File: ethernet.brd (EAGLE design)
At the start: 32.5 x 17 mm, 2 parts, among them CN1 8P8C, CN7 Mini Displayport

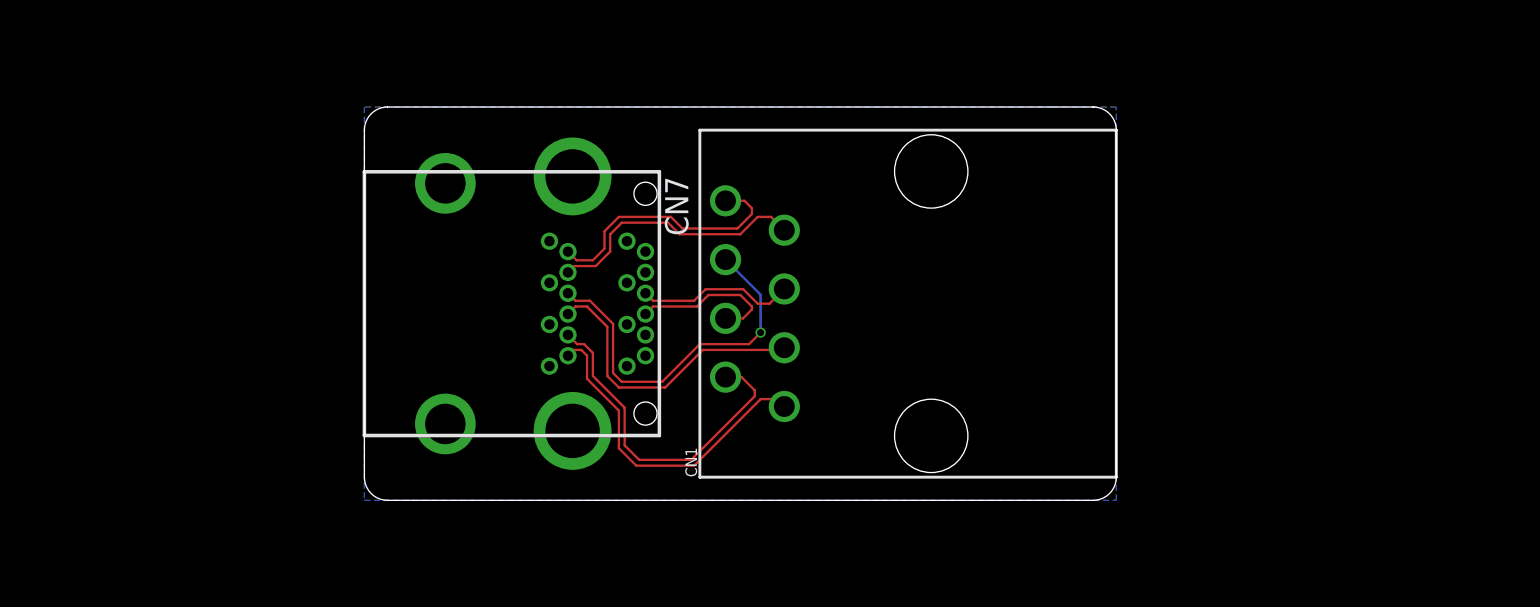
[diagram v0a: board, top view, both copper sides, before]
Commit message: Addition of an ethernet adapter PCB
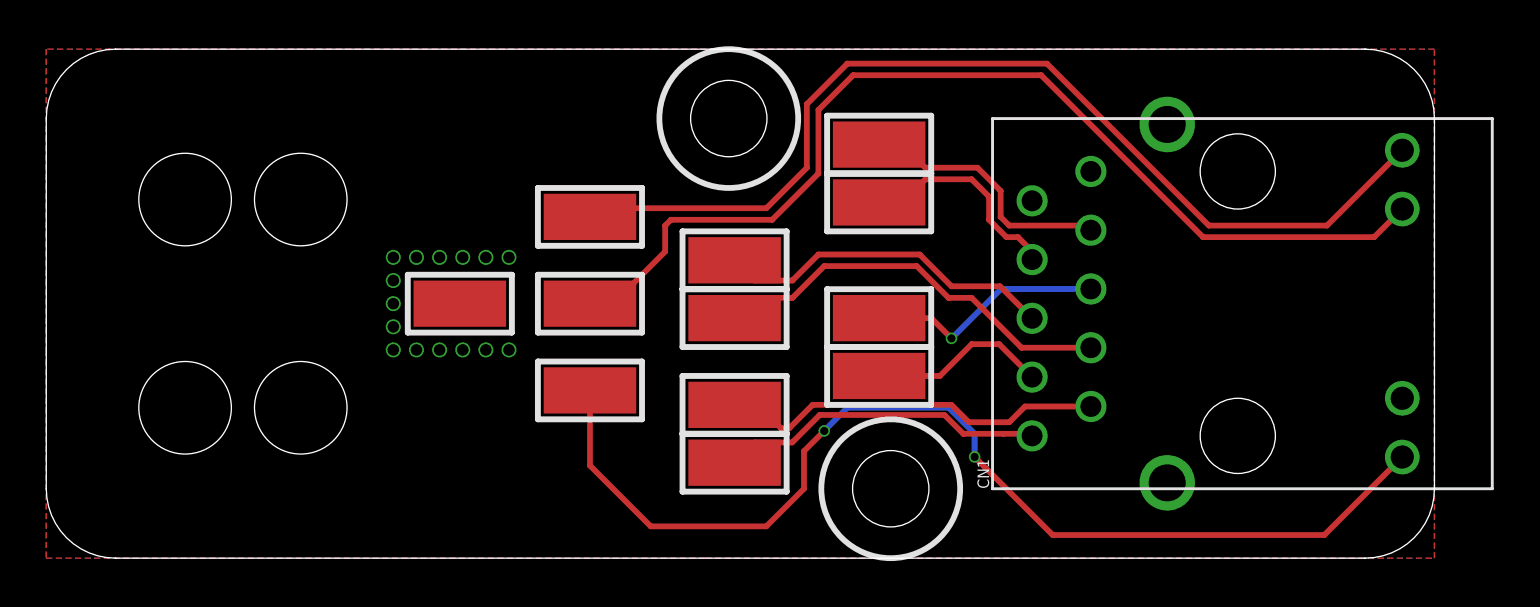
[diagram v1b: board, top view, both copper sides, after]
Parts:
- removed CN7: Mini Displayport, CONNECTORs:2129320-3
- added MECH1, MECH2: 6mm x 3mm, MISC:MOUNTHOLE_6X3
- added TP1, TP10, TP11, TP12, TP2, TP3, TP4, TP5, TP6, TP7, TP8, TP9: TEST_POINT_SQUARE, MISC:OSPREY_HSS_PAD
- CN1: value 8P8C -> HFJ11-1G01ERL; device CONNECTORs:MTJ-880X1 -> CONNECTORs:HFJ11-1G
- moved CN1 14.2 mm to (21.5, 0.00)
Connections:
- removed net ETH_TD_0_N: CN1.2, CN7.15
- removed net ETH_TD_0_P: CN1.1, CN7.17
- removed net ETH_TD_1_N: CN1.6, CN7.9
- removed net ETH_TD_1_P: CN1.3, CN7.11
- removed net ETH_TD_2_N: CN1.5, CN7.10
- removed net ETH_TD_2_P: CN1.4, CN7.12
- removed net ETH_TD_3_N: CN1.8, CN7.3
- removed net ETH_TD_3_P: CN1.7, CN7.5
- new net LED_AMBER: CN1.14, TP11.1
- new net LED_GREEN: CN1.11, TP10.1
- new net N$1: CN1.1, TP1.1
- new net N$2: CN1.2, TP2.1
- new net N$3: CN1.3, TP3.1
- new net N$4: CN1.6, TP4.1
- new net N$5: CN1.4, TP5.1
- new net N$6: CN1.5, TP6.1
- new net N$7: CN1.7, TP7.1
- new net N$8: CN1.8, TP8.1
- new net PWR_SYS_3V3: CN1.13, TP9.1
- net GND: now also CN1.10, CN1.12, CN1.SH1, CN1.SH2, TP12.1; no longer CN7.1, CN7.13, CN7.14, CN7.19, CN7.7, CN7.8, CN7.SH1, CN7.SH2, CN7.SH3, CN7.SH4
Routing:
- net LED_GREEN: track 0.00 -> 46.8 mm, vias 0 -> 2
- net PWR_SYS_3V3: track 0.00 -> 44.9 mm
- net LED_AMBER: track 0.00 -> 43.7 mm
- net N$5: track 0.00 -> 17.8 mm
- net N$2: track 0.00 -> 16.8 mm
- net ETH_TD_1_N: track 15.8 -> 0.00 mm, vias 1 -> 0
- net N$6: track 0.00 -> 14.8 mm
- net ETH_TD_0_N: track 14.7 -> 0.00 mm
- net ETH_TD_0_P: track 14.4 -> 0.00 mm
- net N$1: track 0.00 -> 14.1 mm
- net ETH_TD_1_P: track 12.9 -> 0.00 mm
- net ETH_TD_3_P: track 11.4 -> 0.00 mm
- net N$8: track 0.00 -> 11.3 mm
- net ETH_TD_3_N: track 11.3 -> 0.00 mm
- net N$4: track 0.00 -> 10.4 mm, vias 0 -> 1
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- added copper zone on layer 1, net GND
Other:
- board size 32.5 x 17 mm -> 60 x 22 mm
